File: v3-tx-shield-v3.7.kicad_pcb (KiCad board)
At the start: 2 copper layers, 116.8 x 58.4 mm, 109 parts, among them J1 Conn_01x08_Male, J2 Conn_01x02_Male, J3 Conn_01x02_Male, P1 Power, P2 Analog, P3 Digital, P4 Digital

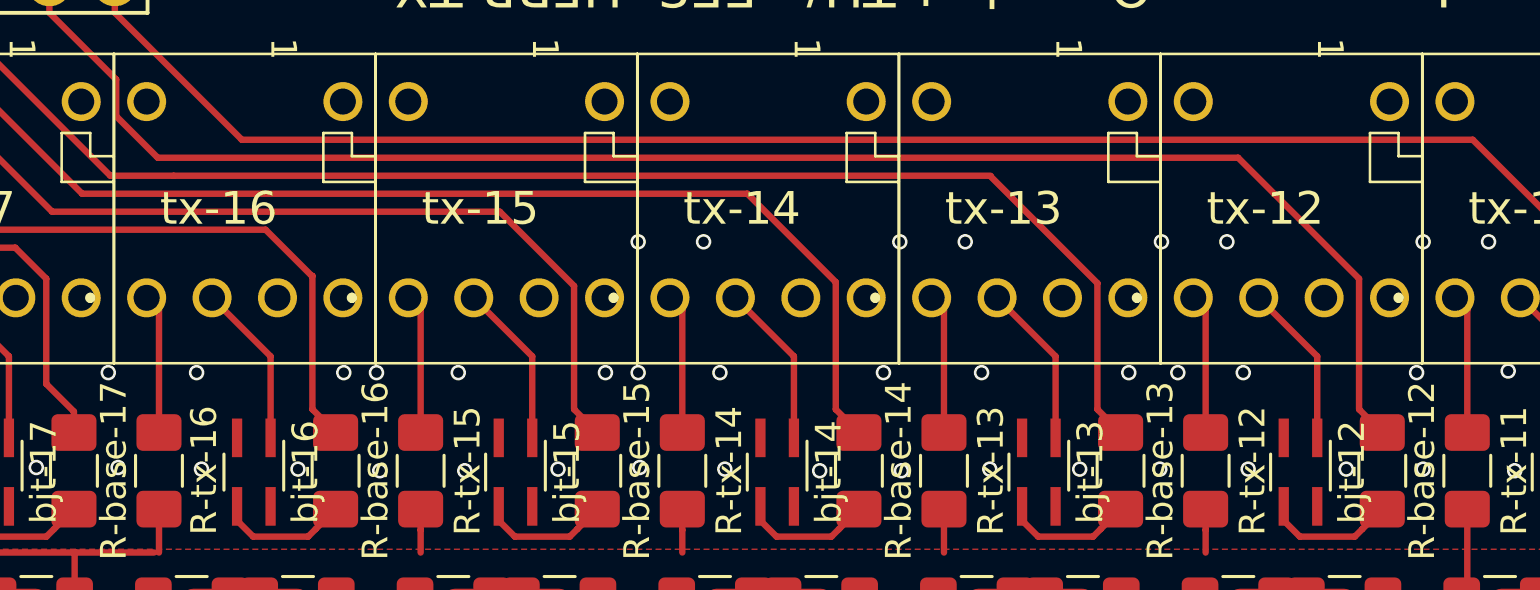
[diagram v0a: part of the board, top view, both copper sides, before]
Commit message: Final version
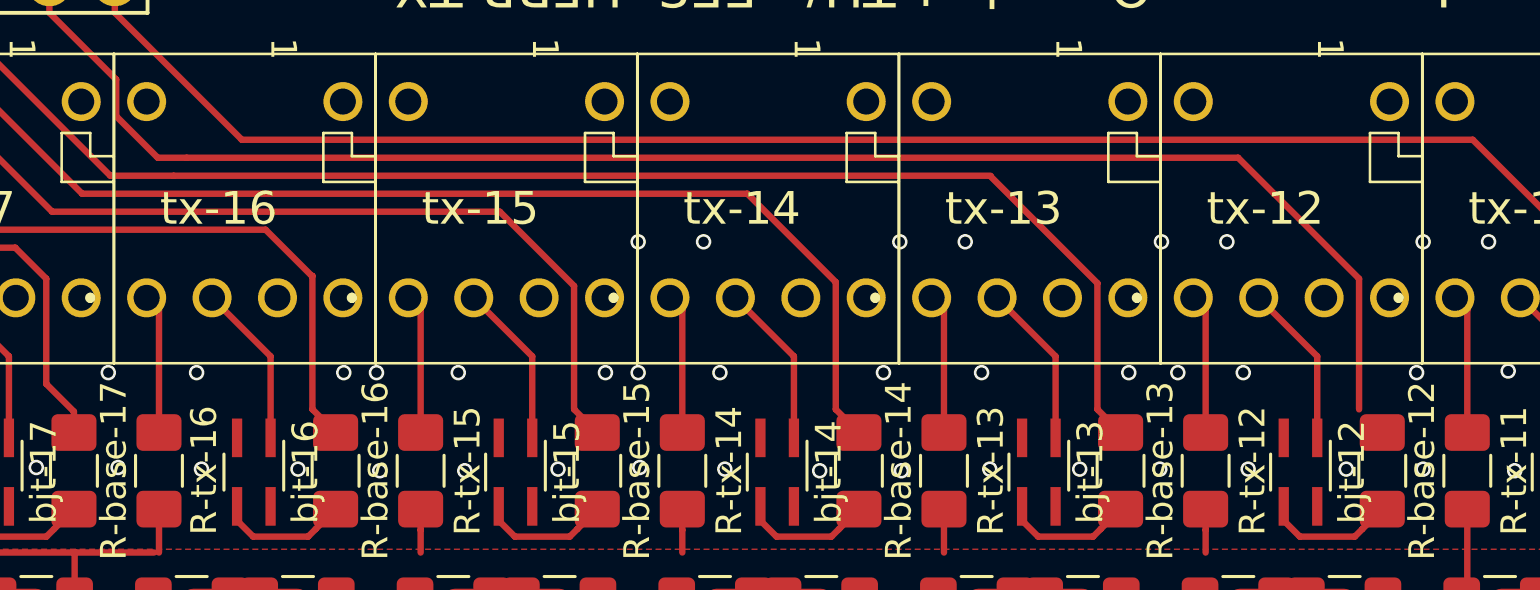
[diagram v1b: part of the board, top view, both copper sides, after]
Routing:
- net sig-1: track 63.6 -> 62.3 mm
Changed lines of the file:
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@@
   (segment (start 176.784 83.1596) (end 208.5036 83.1596) (width 0.25) (layer F.Cu) (net 57))
   (segment (start 212.650998 92.230538) (end 213.5505 93.13004) (width 0.25) (layer F.Cu) (net 57))
-  (segment (start 222.810998 92.230538) (end 223.7105 93.13004) (width 0.25) (layer F.Cu) (net 58))
   (segment (start 222.810998 87.158508) (end 222.810998 92.230538) (width 0.25) (layer F.Cu) (net 58))
+  (segment (start 218.11359 82.4611) (end 222.810998 87.158508) (width 0.25) (layer F.Cu) (net 58))
+  (segment (start 174.550998 79.423998) (end 174.550998 80.8476) (width 0.25) (layer F.Cu) (net 58))
+  (segment (start 174.550998 80.8476) (end 176.164498 82.4611) (width 0.25) (layer F.Cu) (net 58))
   (segment (start 171.958 76.831) (end 174.550998 79.423998) (width 0.25) (layer F.Cu) (net 58))
   (segment (start 171.958 75.565) (end 171.958 76.831) (width 0.25) (layer F.Cu) (net 58))
-  (segment (start 174.550998 79.423998) (end 174.550998 80.8476) (width 0.25) (layer F.Cu) (net 58))
-  (segment (start 174.550998 80.8476) (end 176.164498 82.4611) (width 0.25) (layer F.Cu) (net 58))
-  (segment (start 176.164498 82.4611) (end 218.11359 82.4611) (width 0.25) (layer F.Cu) (net 58))
-  (segment (start 218.11359 82.4611) (end 222.810998 87.158508) (width 0.25) (layer F.Cu) (net 58))
+  (segment (start 177.292 82.4611) (end 218.11359 82.4611) (width 0.25) (layer F.Cu) (net 58))
+  (segment (start 176.164498 82.4611) (end 177.292 82.4611) (width 0.25) (layer F.Cu) (net 58))
   (segment (start 174.498 76.831) (end 174.498 75.565) (width 0.25) (layer F.Cu) (net 59))
   (segment (start 179.4296 81.7626) (end 174.498 76.831) (width 0.25) (layer F.Cu) (net 59))
